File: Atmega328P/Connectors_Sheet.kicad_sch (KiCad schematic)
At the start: 4 parts, among them J1 Conn_01x04_Pin, J2 Conn_01x09_Pin, J3 Conn_01x04_Pin, J4 Conn_02x03_Odd_Even

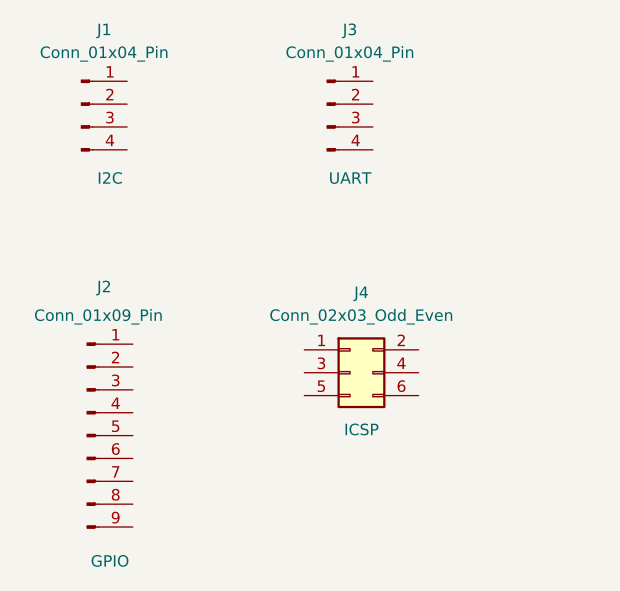
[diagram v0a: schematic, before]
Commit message: Routing completed
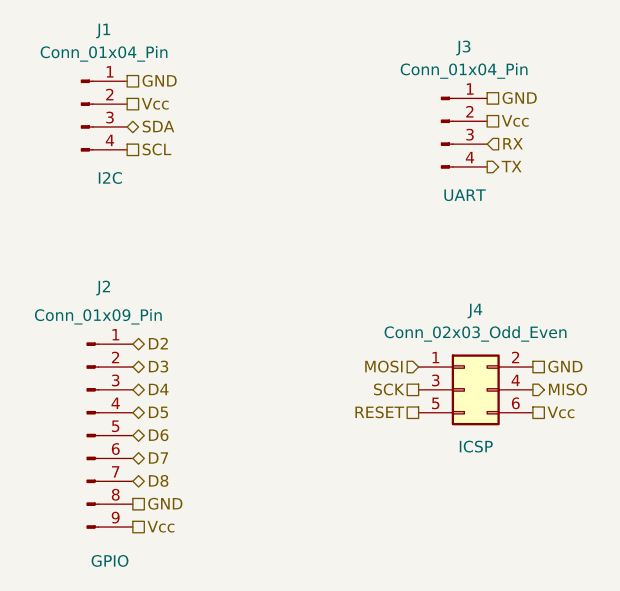
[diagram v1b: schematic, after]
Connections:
- net GND: now reaches J1.1 (Pin_1)
- net GND: now also J2.8 (Pin_8), J3.1 (Pin_1), J4.2 (Pin_2)
- net Vcc: now reaches J1.2 (Pin_2)
- net Vcc: now also J2.9 (Pin_9), J3.2 (Pin_2), J4.6 (Pin_6)
- net SDA: now reaches J1.3 (Pin_3)
- net SCL: now reaches J1.4 (Pin_4)
- net RX: now reaches J3.3 (Pin_3)
- net TX: now reaches J3.4 (Pin_4)
- net D2: now reaches J2.1 (Pin_1)
- net D3: now reaches J2.2 (Pin_2)
- net D4: now reaches J2.3 (Pin_3)
- net D5: now reaches J2.4 (Pin_4)
- net D6: now reaches J2.5 (Pin_5)
- net D7: now reaches J2.6 (Pin_6)
- net D8: now reaches J2.7 (Pin_7)
- net MOSI: now reaches J4.1 (Pin_1)
- net SCK: now reaches J4.3 (Pin_3)
- net MISO: now reaches J4.4 (Pin_4)
- net RESET: now reaches J4.5 (Pin_5)
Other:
- moved on the sheet: J3, J4
